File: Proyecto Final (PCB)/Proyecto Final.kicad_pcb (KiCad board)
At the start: 4 copper layers, 150 x 72 mm, 81 parts, among them IC1 MC9S08MP16xLC, J1 Input, J10 Expansions5, J11 Motor2, J12 Motor4, J13 Expansion2, J14 Luces_LEDs1, J15 Luces_LEDs2, J16 Relay1, J17 Relay3, J18 Relay2, J19 Relay4, J2 DHT11_SENSOR, J20 LCD PINs, J21 Conn_01x04_Male, J3 LDR, J4 TDS_SENSOR, J5 PH_SENSOR, J6 Nivel_L, J7 Motor1, J8 Motor3, J9 Nivel_H, K1 FINDER-36.11, K2 FINDER-36.11, K3 FINDER-36.11, K4 FINDER-36.11, Q1 IRF3205, Q2 IRF3205, SW1 SWDIP, U1 LM358, U10 ULN2003A, U2 LM358, U3 PC817, U4 PC817, U5 MIC4427, U6 ULN2003A, U7 AP63205WU, Y1 Crystal

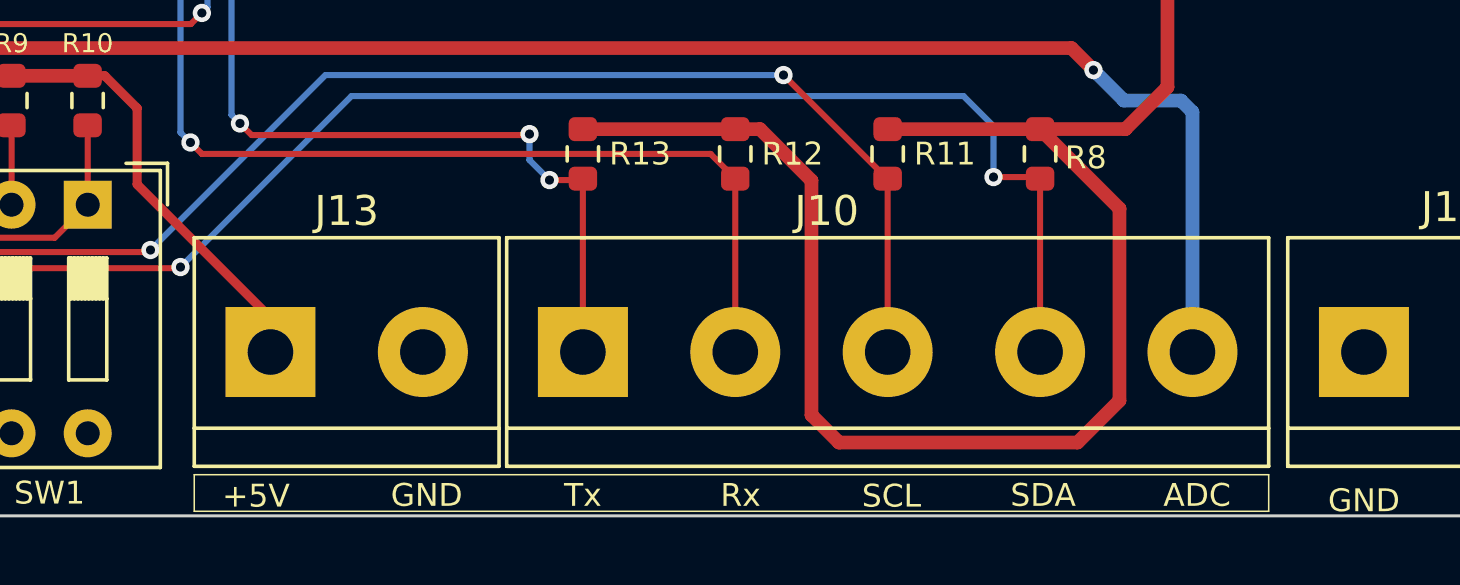
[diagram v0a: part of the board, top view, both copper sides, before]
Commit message: 18:12
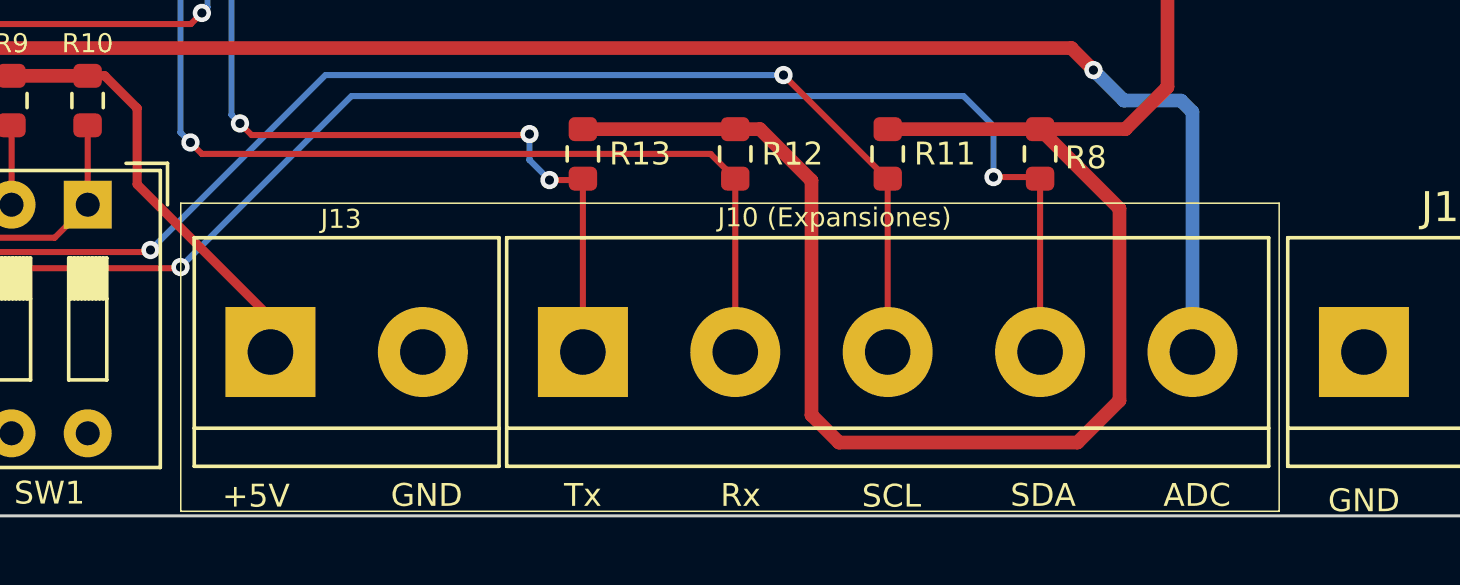
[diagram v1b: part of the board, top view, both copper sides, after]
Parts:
- J10 (Expansiones): renamed from J10
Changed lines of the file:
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@@
     (property "Sheetname" "Expansions")
     (attr through_hole)
-    (fp_text reference "J13" (at 2.54 -4.699) (layer "F.SilkS")
-      (effects (font (size 1 1) (thickness 0.15)))
+    (fp_text reference "J13" (at 2.351 -4.432) (layer "F.SilkS")
+      (effects (font (size 0.635 0.635) (thickness 0.0762)))
     )
     (fp_text value "Expansion2" (at 2.54 5.08) (layer "F.Fab")
@@
     (property "Sheetname" "Expansions")
     (attr through_hole)
-    (fp_text reference "J10" (at 8.128 -4.699) (layer "F.SilkS")
-      (effects (font (size 1 1) (thickness 0.15)))
+    (fp_text reference "J10 (Expansiones)" (at 8.387 -4.482) (layer "F.SilkS")
+      (effects (font (size 0.635 0.635) (thickness 0.0762)))
     )
     (fp_text value "Expansions5" (at 10.15 4.6) (layer "F.Fab")
@@
     )
   )
-  (gr_rect (start 192.659 133.1214) (end 228.473 134.3406) (layer "F.SilkS") (width 0.0508) (fill none))
+  (gr_rect (start 192.209 124.0714) (end 228.823 134.3406) (layer "F.SilkS") (width 0.0508) (fill none))
   (gr_rect (start 91.186 134.493) (end 241.186 62.493) (layer "Edge.Cuts") (width 0.1) (fill none))
   (gr_text "500mA" (at 200.406 63.627) (layer "F.SilkS")
